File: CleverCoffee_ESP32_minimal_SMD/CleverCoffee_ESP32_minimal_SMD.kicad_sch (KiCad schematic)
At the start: 30 parts

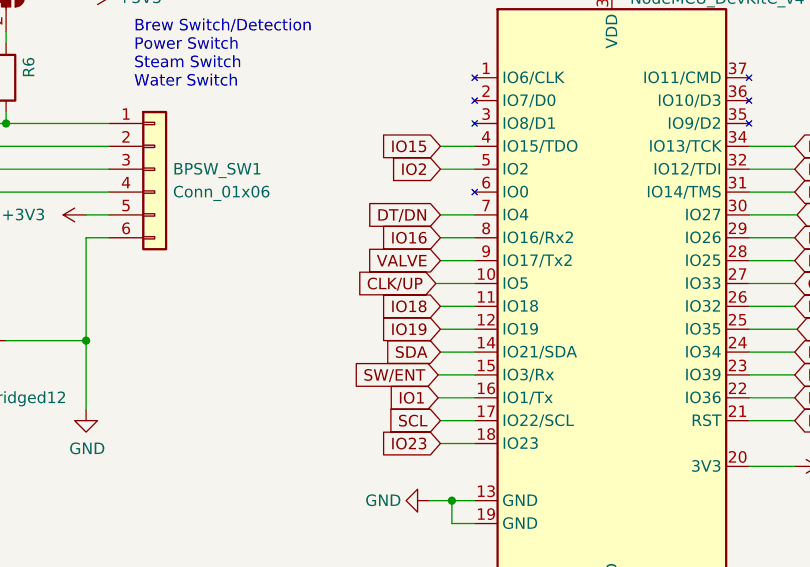
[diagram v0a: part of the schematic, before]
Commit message: draft pcb layout
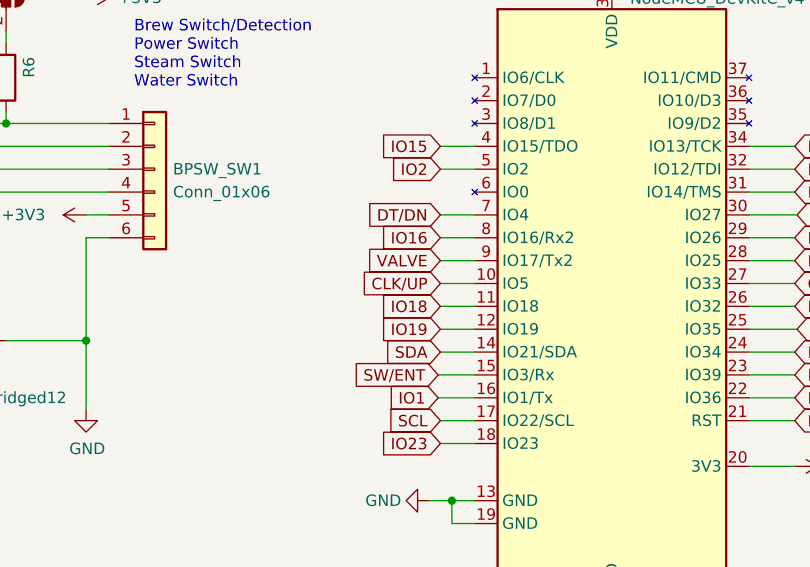
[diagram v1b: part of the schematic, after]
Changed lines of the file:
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@@
 	(wire
 		(pts
-			(xy 226.822 63.5) (xy 231.14 63.5)
-		)
-		(stroke
-			(width 0)
-			(type default)
-		)
-	)
-	(wire
-		(pts
 			(xy 227.33 68.58) (xy 231.14 68.58)
 		)
@@
 	(wire
 		(pts
+			(xy 227.33 63.5) (xy 231.14 63.5)
+		)
+		(stroke
+			(width 0)
+			(type default)
+		)
+	)
+	(wire
+		(pts
 			(xy 261.62 76.2) (xy 266.7 76.2)
 		)
@@
 	(global_label "CLK/UP"
 		(shape input)
-		(at 226.822 63.5 180)
+		(at 227.33 63.5 180)
 		(fields_autoplaced yes)
 		(effects
@@
 		)
 		(property "Intersheetrefs" "${INTERSHEET_REFS}"
-			(at 221.2641 63.4206 0)
+			(at 221.7721 63.4206 0)
 			(hide yes)
 			(show_name no)
@@
 	)
 	(symbol
+		(lib_name "+3.3V_1")
 		(lib_id "power:+3.3V")
 		(at 266.7 83.82 270)
@@
 			)
 		)
-		(property "Description" ""
+		(property "Description" "Power symbol creates a global label with name \"+3.3V\""
 			(at 266.7 83.82 0)
 			(hide yes)
